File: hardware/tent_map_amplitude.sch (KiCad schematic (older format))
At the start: 40 parts, among them U1 LM339AN, U2 TL082IP, U3 TL082IP

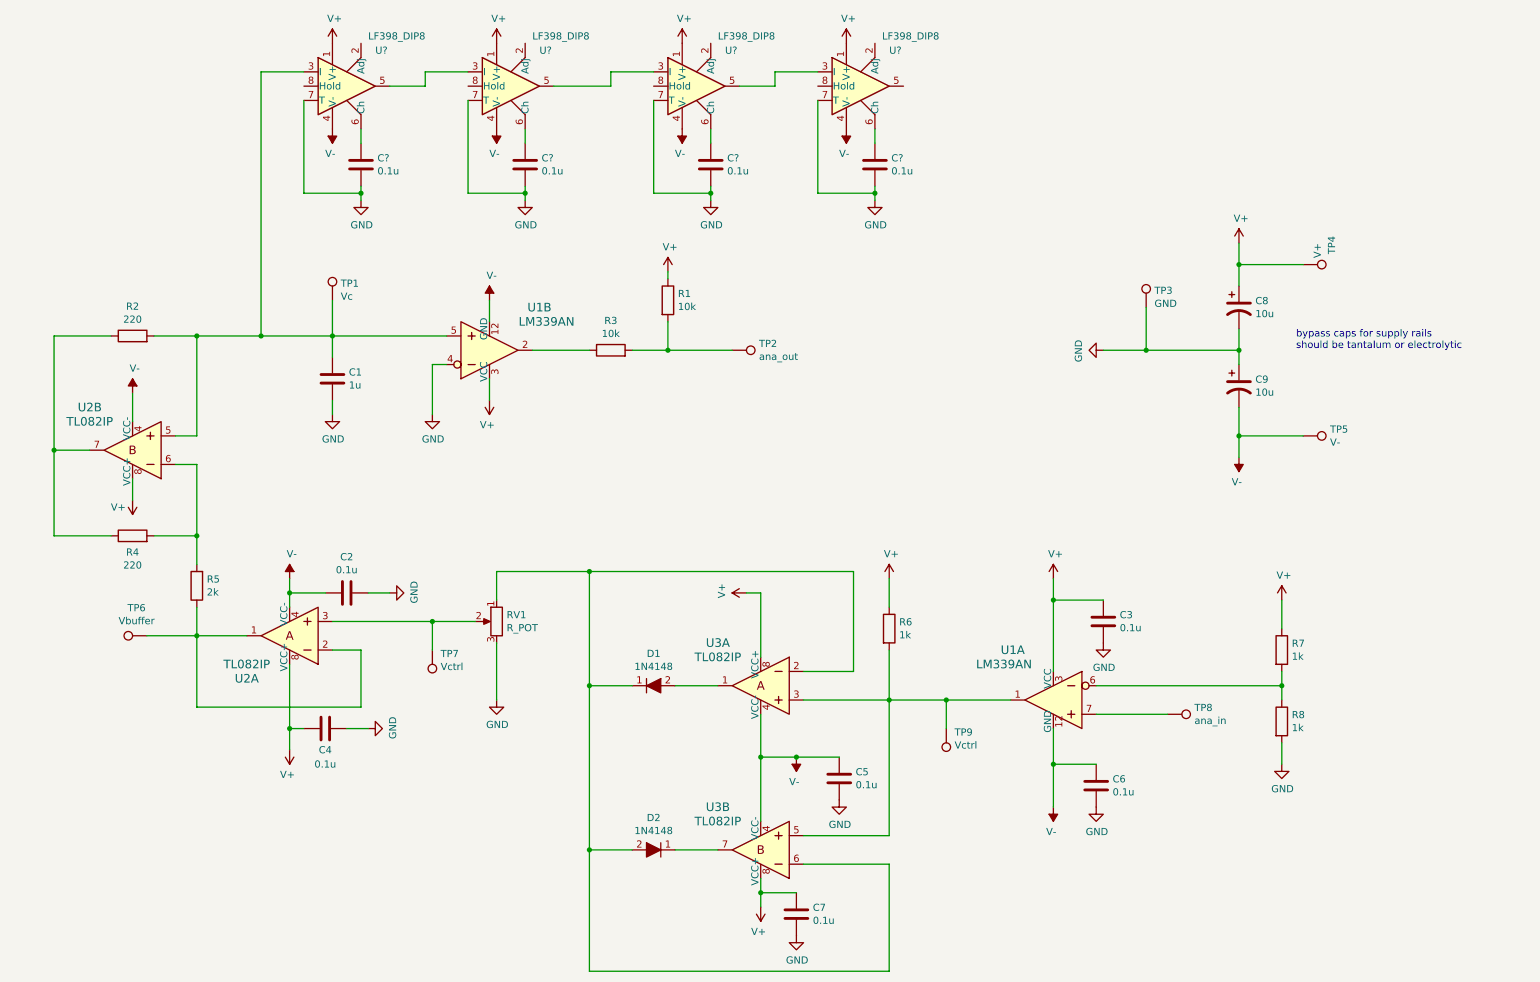
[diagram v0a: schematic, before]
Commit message: Complete PCB (unreviewed)
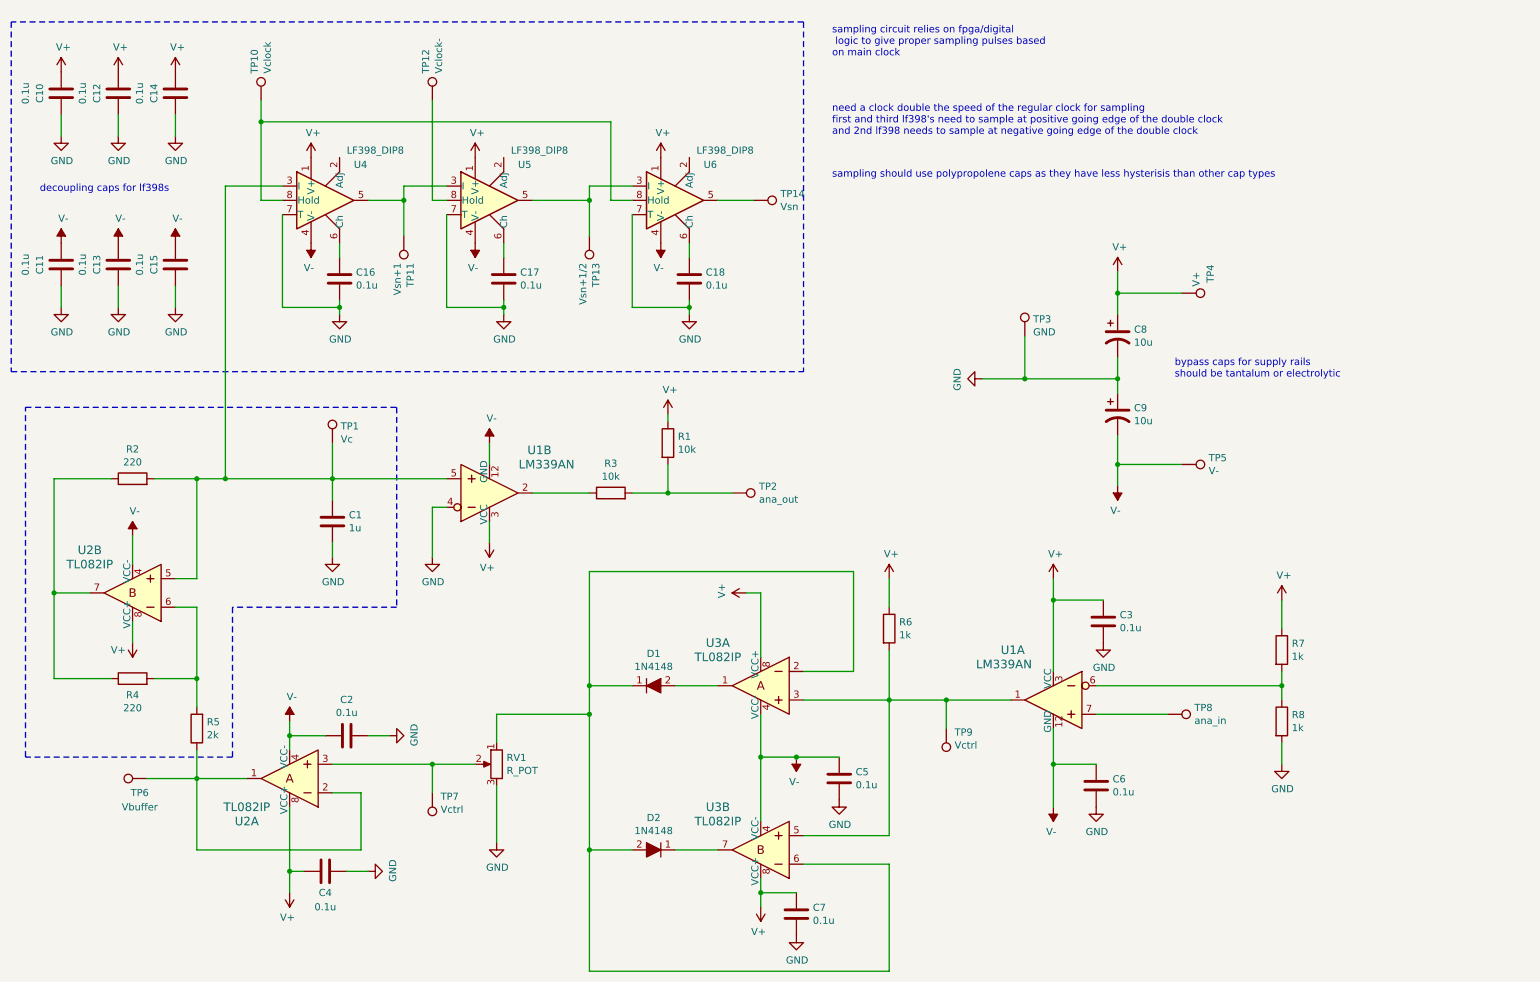
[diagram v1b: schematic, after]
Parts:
- removed C?: 0.1u, Capacitor_SMD:C_0805_2012Metric_Pad1.18x1.45mm_HandSolder, symbol Device:C
- removed U?: LF398_DIP8, symbol Analog:LF398_DIP8
- added C10, C11, C12, C13, C14, C15: 0.1u, Capacitor_SMD:C_0805_2012Metric_Pad1.18x1.45mm_HandSolder, symbol Device:C
- added TP10: Vclock, TestPoint:TestPoint_Bridge_Pitch2.54mm_Drill1.0mm, symbol Connector:TestPoint
- added TP11: Vsn+1, TestPoint:TestPoint_Bridge_Pitch2.54mm_Drill1.0mm, symbol Connector:TestPoint
- added TP12: Vclock-, TestPoint:TestPoint_Bridge_Pitch2.54mm_Drill1.0mm, symbol Connector:TestPoint
- added TP13: Vsn+1/2, TestPoint:TestPoint_Bridge_Pitch2.54mm_Drill1.0mm, symbol Connector:TestPoint
- added TP14: Vsn, TestPoint:TestPoint_Bridge_Pitch2.54mm_Drill1.0mm, symbol Connector:TestPoint
- C16, C17, C18: renamed from C?; footprint Capacitor_SMD:C_0805_2012Metric_Pad1.18x1.45mm_HandSolder -> Capacitor_THT:C_Rect_L10.3mm_W5.0mm_P7.50mm_MKS4
- U4, U5, U6: renamed from U?; footprint (none) -> digikey-footprints:DIP-8_W7.62mm
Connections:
- net GND: now also C10.1, C11.1, C12.1, C13.1, C14.1, C15.1
- net V+: now also C10.2, C12.2, C14.2
- net V-: now also C11.2, C13.2, C15.2
- net at U4.5, U5.3 (I): now also TP11.1
- net at U5.5, U6.3 (I): now also TP13.1
- net at U5.8 (Hold): now also TP12.1
- net at U4.8 (Hold): now also U6.8 (Hold), TP10.1
- net at U6.5: now also TP14.1
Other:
- note added: "decoupling caps for lf398s\n"
- note added: "need a clock double the speed of the regular clock for sampling\nfirst and third lf398's need to sample at positive going edge of the double clock\nand 2nd lf398 needs to sample at negative going edge of the double clock"
- note added: "sampling circuit relies on fpga/digital\n logic to give proper sampling pulses based \non main clock"
- note added: "sampling should use polypropolene caps as they have less hysterisis than other cap types\n"
- moved on the sheet: C1, C16, C17, C18, C2, C4, C8, C9, R1, R2, R3, R4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
